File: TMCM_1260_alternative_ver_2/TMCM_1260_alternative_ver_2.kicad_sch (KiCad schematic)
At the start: 110 parts, among them J1 Motor, J2 CAN, J3 I/O, J4 Power, J5 USB_B_Micro, J6 JXD2-0Z10NL, J7 Conn_01x05, Q1 NVMFD5C650NLT1G, Q2 NVMFD5C650NLT1G, Q3 NVMFD5C650NLT1G, Q4 NVMFD5C650NLT1G, U1 LMZM23600V3SILR, U2 STM32F091CCTx, U3 TCAN337, U4 TMC5160A-TA-T, U5 AS5047P-ATSM, U6 STM32H563RGTx, U7 CP2102N-Axx-xQFN24, U8 TMC4361A-LA-T, U9 LAN8742A-CZ-TR, Y1 Crystal_Small

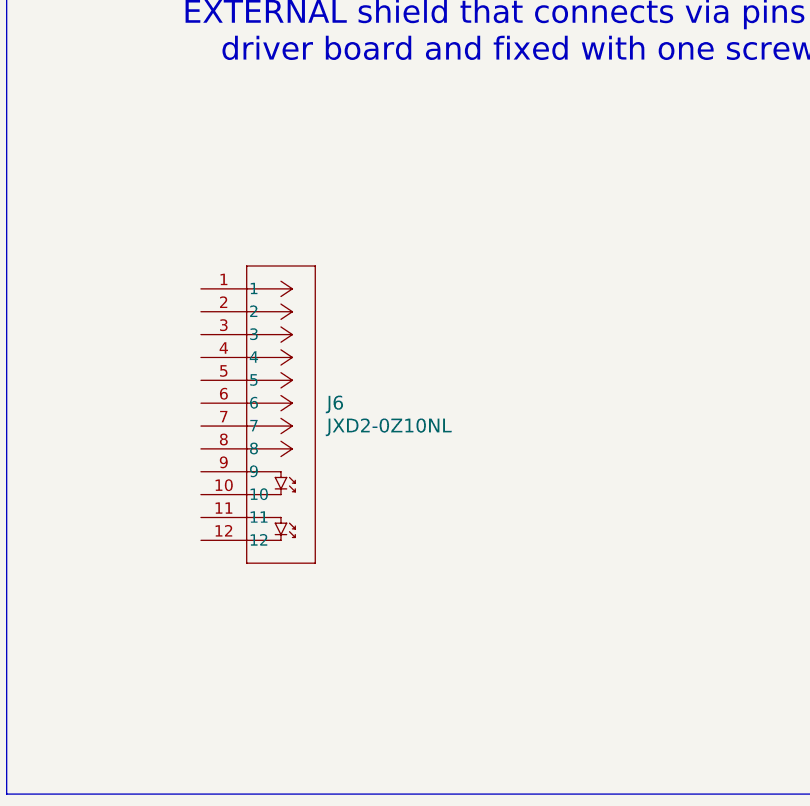
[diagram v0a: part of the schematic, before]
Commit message: upload
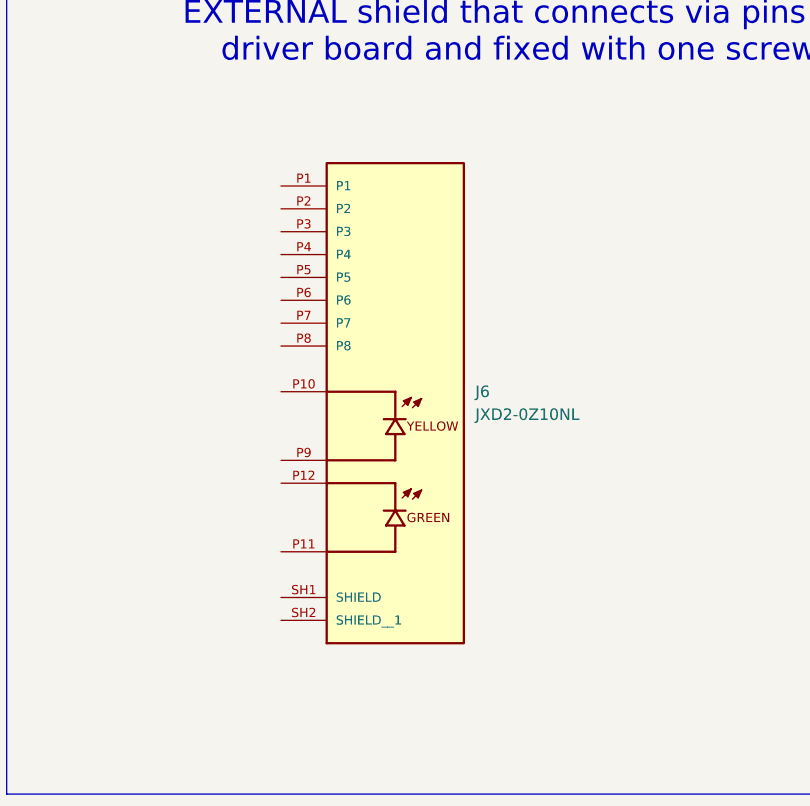
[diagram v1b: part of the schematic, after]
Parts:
- removed J6: JXD2-0Z10NL, JXD2_0Z10NL:JXD2_0Z10NL, symbol JXD2_0Z10NL:JXD2-0Z10NL
- added J6: JXD2-0Z10NL, JXD2_0Z10NL:JXD2_0Z10NL, symbol JXD2-0Z10NL:JXD2-0Z10NL

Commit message: tmc4361 added ver_2
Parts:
- removed U2: STM32F091CCTx, Package_QFP:LQFP-48_7x7mm_P0.5mm, symbol MCU_ST_STM32F0:STM32F091CCTx
- removed Y1: Crystal_Small, digikey-footprints:SMD-2_3.2x2.5mm, symbol Device:Crystal_Small
- added C44, C45: 2.2u, Capacitor_SMD:C_0603_1608Metric_Pad1.08x0.95mm_HandSolder, symbol Device:C
- added C46: 4.7u, Capacitor_SMD:C_0603_1608Metric_Pad1.08x0.95mm_HandSolder, symbol Device:C
- added C47, C48: 15p, Capacitor_SMD:C_0603_1608Metric, symbol Device:C
- added C49, C57, C58, C59, C60, C61, C62: 0.1u, Capacitor_SMD:C_0603_1608Metric_Pad1.08x0.95mm_HandSolder, symbol Device:C
- added C50: 470p, Capacitor_SMD:C_0603_1608Metric_Pad1.08x0.95mm_HandSolder, symbol Device:C
- added C51: 1u, Capacitor_SMD:C_0603_1608Metric_Pad1.08x0.95mm_HandSolder, symbol Device:C
- added C52, C53, C54, C56: 10pF, Capacitor_SMD:C_0603_1608Metric_Pad1.08x0.95mm_HandSolder, symbol Device:C
- added C55: 0.022uF, Capacitor_SMD:C_0603_1608Metric_Pad1.08x0.95mm_HandSolder, symbol Device:C
- added R36, R37: 330, Resistor_SMD:R_0603_1608Metric, symbol Device:R_Small
- added R38, R42, R43, R44: 49.9, Resistor_SMD:R_0603_1608Metric, symbol Device:R_Small
- added R45, R46, R47: 100, Resistor_SMD:R_0603_1608Metric, symbol Device:R_Small
- added Y2: 25Mhz, Crystal:Crystal_SMD_2016-4Pin_2.0x1.6mm, symbol Device:Crystal_GND24_Small
- C24: now not fitted; now left out of the parts list
- C5, C6: value 4.3p -> 0.1u; footprint Capacitor_SMD:C_0603_1608Metric -> Capacitor_SMD:C_0603_1608Metric_Pad1.08x0.95mm_HandSolder; PN GRM1885C1H4R3BA01D -> CL10B104KO8NNNC
- R32: value 4k7 -> 12.1k; PN ERJ-3EKF4701V -> RC0603FR-0712K4L; now fitted
- R33: value 4k7 -> 10k; footprint Resistor_SMD:R_0603_1608Metric_Pad0.98x0.95mm_HandSolder -> Resistor_SMD:R_0603_1608Metric; PN ERJ-3EKF4701V -> (none); now fitted
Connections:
- net SPI2_MISO is gone; now on net SDI_ENC: U5.3 (MISO)
- net SPI2_MOSI is gone; now on net SDO_ENC: U5.4 (MOSI)
- net SPI2_NSS is gone; now on net NSCS_ENC: U5.1 (CSn)
- net SPI2_SCK is gone; now on net SCLK_ENC: U5.2 (CLK)
- net +3V3: now also J6.P2, J6.P5, R33.1, U6.1 (VBAT), U6.13 (VDDA), U6.19 (VDD), U6.32 (VDD), U6.48 (VDD), U6.64 (VDD), U8.19 (NFREEZE), U8.26 (VCC), U8.37 (VCC), U8.5 (VCC), U9.1 (VDD2A), U9.19 (VDD1A), U9.9 (VDDIO), C46.1, C52.2, C53.2, C54.2, C55.2, C56.2, C57.1, C58.1, C59.1, C60.2, R38.1, R42.1, R43.1, R44.1; no longer R32.2, R33.2
- net CSN: now also U6.58 (PB6), U8.2 (NSCSIN); no longer U4.13 (CSN_CFG3)
- net DRV_ENN: now also U6.27 (PB1)
- net GND: now also C6.1, J6.P8, J6.SH1 (SHIELD), J6.SH2 (SHIELD__1), R32.1, U6.12 (VSSA), U6.18 (VSS), U6.31 (VSS), U6.47 (VSS), U6.60 (BOOT0), U6.63 (VSS), U8.15 (GND), U8.25 (GND), U8.34 (TEST_MODE), U8.36 (GND), U8.6 (GND), U9.25 (EPAD), C44.1, C45.2, C46.2, C47.1, C48.1, C49.2, C50.2, C51.2, C52.1, C53.1, C54.1, C55.1, C56.1, C57.2, C58.2, C59.2, C60.1, C61.1, C62.1, R36.2, R37.2, Y2.2, Y2.4; no longer C6.2
- net NRST: now also U6.7 (NRST)
- net ON_INDICATOR: now also U6.11 (PC3)
- net Out_1: now also C5.1, U8.12 (STOPL)
- net Out_2: now also C6.2, U8.14 (STOPR)
- net RXD: now also U6.44 (PA11)
- net SCK: now also U6.55 (PB3(JTDO), U8.3 (SCKIN); no longer U4.14 (SCK_CFG2)
- net SENSOR_INDICATOR: now also U6.10 (PC2)
- net SPI_MISO: now also U6.56 (PB4(NJTRST)), U8.7 (SDOIN); no longer U4.16 (SDO_CFG0)
- net SPI_MOSI: now also U6.57 (PB5), U8.4 (SDIIN); no longer U4.15 (SDI_CFG1)
- net SWCLK: now also U6.49 (PA14(JTCK)
- net SWDIO: now also U6.46 (PA13(JTMS)
- net TXD: now also U6.45 (PA12)
- net UART_RX: now also U6.43 (PA10)
- net UART_TX: now also U6.42 (PA9)
- net TXP: now reaches J6.P1
- net TXP: now also U9.21 (TXP), R42.2
- net at J6.P10: now also R36.1
- net LED2: now reaches J6.P11
- net LED2: now also U9.2 (LED2/NINT/NPME/*NINTSEL)
- net at J6.P12: now also R37.1
- net TXN: now reaches J6.P3
- net TXN: now also U9.20 (TXN), R38.2
- net RXP: now reaches J6.P4
- net RXP: now also U9.23 (RXP), R44.2
- net RXN: now reaches J6.P6
- net RXN: now also U9.22 (RXN), R43.2
- net LED1: now reaches J6.P9
- net LED1: now also U9.3 (LED1/NINT/NPME/*REGOFF)
- net at U9.11 (CRS_DV/*MODE2): now also R47.1
- net ETH_MDIO: now reaches U9.12 (MDIO)
- net ETH_MDIO: now also U6.16 (PA2)
- net ETH_MDC: now reaches U9.13 (MDC)
- net ETH_MDC: now also U6.9 (PC1)
- net ETH_REF_CLK: now reaches U9.14 (NINT/REFCLKO)
- net ETH_REF_CLK: now also U6.15 (PA1)
- net LAN_NRST: now reaches U9.15 (NRST)
- net LAN_NRST: now also R33.2, U6.17 (PA3), C49.1
- net ETH_TX_EN: now reaches U9.16 (TXEN)
- net ETH_TX_EN: now also U6.21 (PA5)
- net ETH_TXD0: now reaches U9.17 (TXD0)
- net ETH_TXD0: now also U6.33 (PB12)
- net ETH_TXD1: now reaches U9.18 (TXD1)
- net ETH_TXD1: now also U6.36 (PB15)
- net at U9.24 (RBIAS): now also R32.2
- net CLKIN: now reaches U9.5 (XTAL1/CLKIN)
- net CLKIN: now also U6.40 (PC9)
- net VDDCR: now reaches U9.6 (VDDCR)
- net VDDCR: now also C50.1, C51.1
- net at U9.7 (RXD1/*MODE1): now also R45.1
- net at U9.8 (RXD0/*MODE0): now also R46.1
- net ETH_CRS_DV: now reaches U6.23 (PA7)
- net ETH_CRS_DV: now also R47.2
- net ETH_RXD0: now reaches U6.24 (PC4)
- net ETH_RXD0: now also R46.2
- net ETH_RXD1: now reaches U6.25 (PC5)
- net ETH_RXD1: now also R45.2
- net TARGET_REACHED: now reaches U6.26 (PB0)
- net TARGET_REACHED: now also U8.31 (TARGET_REACHED)
- net INTR: now reaches U6.28 (PB2)
- net INTR: now also U8.33 (INTR)
- net at U6.30 (VCAP): now also U6.62 (VCAP), C44.2, C45.1
- net CLK_EXT: now reaches U6.41 (PA8)
- net CLK_EXT: now also U8.38 (CLK_EXT)
- net at U6.5 (PH0): now also C47.2, Y2.3
- net at U6.6 (PH1): now also C48.2, Y2.1
- net NSCS_ENC: now reaches U8.1 (ANEG_NSCLK)
- net SDI_ENC: now reaches U8.10 (B_SDI)
- net SDO_ENC: now reaches U8.11 (BNEG_NSDI)
- net at U8.16 (VDD1V8): now also C62.2
- net SPI_MOSI_DRV: now reaches U8.27 (SDODRV_SCLK)
- net SPI_MOSI_DRV: now also U4.15 (SDI_CFG1)
- net SPI_MISO_DRV: now reaches U8.28 (SDIDRV_NSCLK)
- net SPI_MISO_DRV: now also U4.16 (SDO_CFG0)
- net SCK_DRV: now reaches U8.29 (SCKDRV_NSDO)
- net SCK_DRV: now also U4.14 (SCK_CFG2)
- net CSN_DRV: now reaches U8.30 (NSCSDRV_SDO)
- net CSN_DRV: now also U4.13 (CSN_CFG3)
- net at U8.35 (VDD1V8): now also C61.2
- net SCLK_ENC: now reaches U8.40 (A_SCLK)
- no-connect marks 31 -> 32
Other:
- note added: "Search: LAN8742 RMII PHY Customer Evaluation Board Schematic"
- note added: "exposed pad must be connected to the ground plane with a via array."
- note removed: "will be migrating to STM32H563RGT6"
- moved on the sheet: C10, C2, C36, C37, C39, C7, C8, J6, U5, U6, U8, U9
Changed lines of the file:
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@@
 	(generator "eeschema")
 	(generator_version "8.0")
-	(paper "A2")
+	(paper "A1")
